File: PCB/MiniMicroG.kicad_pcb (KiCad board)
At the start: 2 copper layers, 111.9 x 88.1 mm, 21 parts, among them J1 .91"OLED, SW1 CHERRY_MX, SW2 CHERRY_MX, SW4 CHERRY_MX, SW5 CHERRY_MX, SW6 CHERRY_MX, SW7 RotaryEncoder_Switch, SW8 CHERRY_MX, U1 XIAO-RP2040-DIP

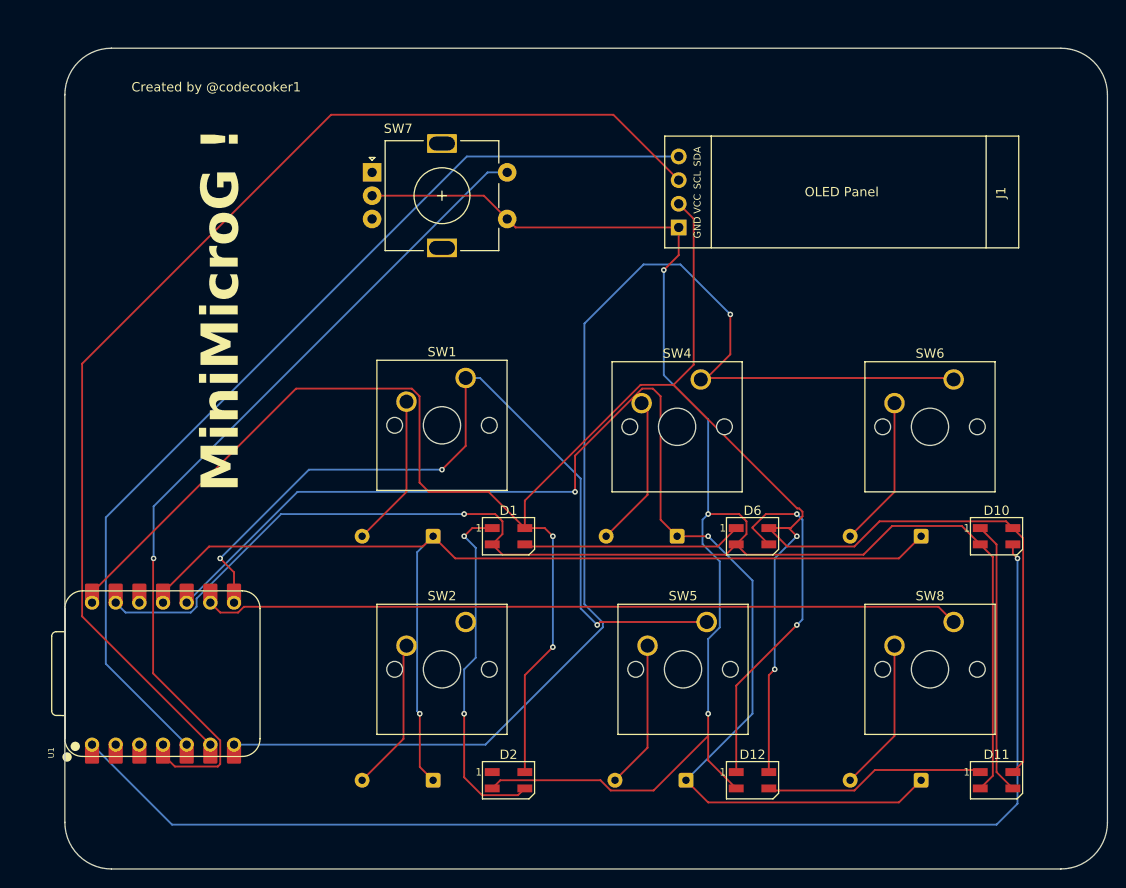
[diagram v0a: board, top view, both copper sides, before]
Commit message: Update PCB
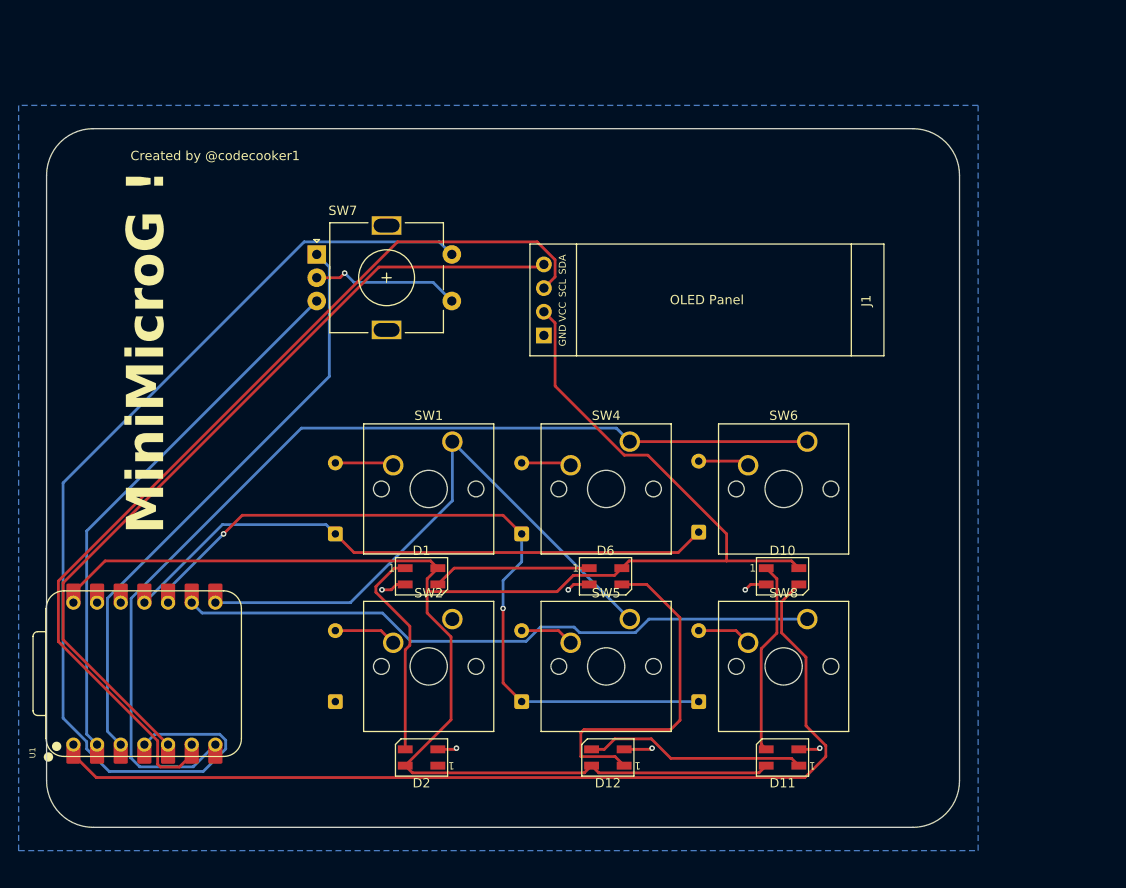
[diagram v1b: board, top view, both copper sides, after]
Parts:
- moved D9 25.3 mm to (149.0, 113.0), turned to 90 degrees
- moved D3 23.9 mm to (149.0, 94.8), turned to 90 degrees
- moved D10 23.4 mm to (158.0, 99.5)
- moved D11 23.1 mm to (158.0, 119.0), turned to 180 degrees
- moved D8 19.6 mm to (130.0, 113.0), turned to 90 degrees
- moved J1 18.5 mm to (168.9, 75.9)
- moved SW6 17.1 mm to (160.7, 85.1)
- moved D7 16.7 mm to (130.0, 95.0), turned to 90 degrees
- moved D6 16.4 mm to (139.0, 99.5)
- moved D12 15.7 mm to (139.2, 119.0), turned to 180 degrees
- moved SW8 15.7 mm to (160.7, 104.1)
- moved D5 13.5 mm to (110.0, 113.0), turned to 90 degrees
- moved SW7 10.6 mm to (108.0, 65.0)
- moved D4 10.5 mm to (110.0, 95.0), turned to 90 degrees
- moved D1 10.3 mm to (119.2, 99.5)
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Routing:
- net GND: track 267.0 -> 31.1 mm, vias 4 -> 7
- net +5V: track 252.8 -> 184.7 mm, vias 4 -> 0
- net Net-(U1-GPIO28/ADC2/A2): track 0.00 -> 63.6 mm
- net Net-(U1-GPIO27/ADC1/A1): track 0.00 -> 58.3 mm
- net Net-(D7-K): track 140.4 -> 82.2 mm
- net Net-(D3-K): track 114.6 -> 65.1 mm, vias 1 -> 0
- net Net-(D10-DIN): track 131.9 -> 105.0 mm, vias 1 -> 0
- net Net-(U1-GPIO1/RX): track 89.2 -> 63.3 mm, vias 3 -> 0
- net Net-(U1-GPIO0/TX): track 133.1 -> 108.4 mm, vias 1 -> 0
- net Net-(J1-Pin_3): track 124.6 -> 102.2 mm
- net Net-(U1-GPIO29/ADC3/A3): track 91.3 -> 109.9 mm, vias 1 -> 0
- net Net-(J1-Pin_4): track 105.5 -> 87.8 mm
- net Net-(D1-DOUT): track 37.9 -> 23.2 mm, vias 2 -> 0
- net Net-(U1-GPIO2/SCK): track 81.2 -> 69.3 mm
- net Net-(D3-A): track 16.4 -> 5.49 mm
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- added copper zone on B.Cu, net GND
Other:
- board size 111.9 x 88.1 mm -> 98 x 75 mm
